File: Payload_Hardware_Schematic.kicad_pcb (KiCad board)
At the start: 2 copper layers, 109 x 54.5 mm, 10 parts, among them J1 Micro_SD_Card, J2 Conn_01x02_Socket, J3 Conn_01x04_Pin, J4 Conn_01x02, J5 Conn_01x04_Pin, U1 STM32F411 BlackPill, U2 MPM3610, U4 LSM9DS1, U5 MPM3610, U6 BMP388

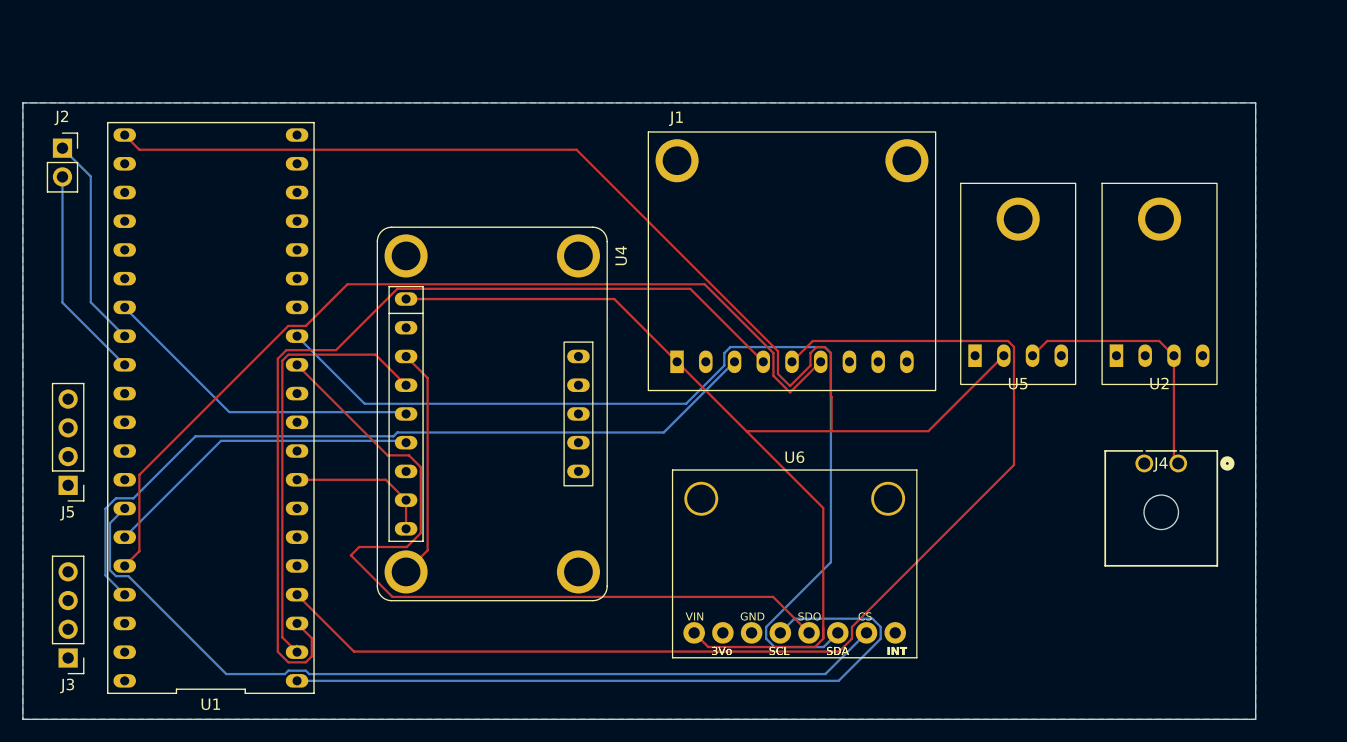
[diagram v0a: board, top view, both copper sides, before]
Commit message: PCB Layout 2
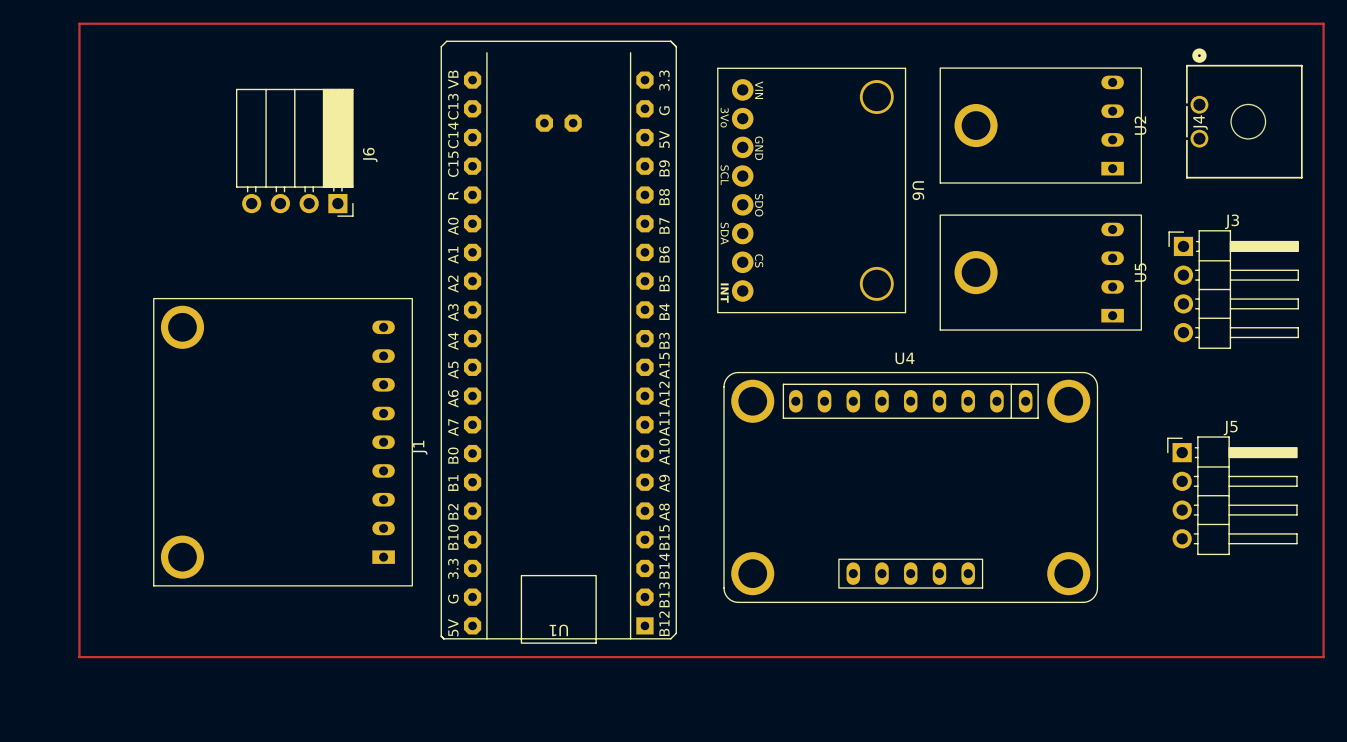
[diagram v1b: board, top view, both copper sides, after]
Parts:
- removed J2: Conn_01x02_Socket, Connector_PinSocket_2.54mm:PinSocket_1x02_P2.54mm_Vertical
- added J6: Conn_01x04_Socket, Connector_PinSocket_2.54mm:PinSocket_1x04_P2.54mm_Horizontal, F.Cu at (92.8, 56.4)
- J3, J5: footprint Connector_PinHeader_2.54mm:PinHeader_1x04_P2.54mm_Vertical -> Connector_PinHeader_2.54mm:PinHeader_1x04_P2.54mm_Horizontal
- U1: footprint Avionics_Symbols:STM32F411 -> Payload-STM32:STM32F411_Black_Pill
- moved J3 105.1 mm to (167.6, 60.2), turned to 0 degrees
- moved J5 98.5 mm to (167.5, 78.4), turned to 0 degrees
- moved U4 44.6 mm to (143.5, 73.9), turned to 180 degrees
- moved J1 36.8 mm to (96.9, 77.5), turned to 90 degrees
- moved U6 33.1 mm to (134.7, 55.2), turned to -90 degrees
- moved J4 31.8 mm to (169.0, 47.7), turned to 90 degrees
- moved U1 31.1 mm to (112.4, 69.6), turned to 180 degrees
- moved U2 20.8 mm to (161.3, 49.5), turned to 90 degrees
- moved U5 11.1 mm to (161.3, 62.5), turned to 90 degrees
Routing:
- net /<NO NET>: track 176.9 -> 0.00 mm
- net /MOSI2: track 104.0 -> 0.00 mm
- net /MOSI3: track 87.4 -> 0.00 mm
- net /NSS2: track 82.1 -> 0.00 mm
- net /MISO2: track 81.1 -> 0.00 mm
- net /NSS3: track 78.4 -> 0.00 mm
- net /MISO3: track 71.1 -> 0.00 mm
- net /SCK2: track 69.3 -> 0.00 mm
- net /SCK3: track 63.9 -> 0.00 mm
- net /SCK4: track 39.2 -> 0.00 mm
- net /MOSI4: track 28.8 -> 0.00 mm
- net /CSIMU: track 28.5 -> 0.00 mm
- net /7.2V: track 23.3 -> 0.00 mm
- net /GND: track 20.9 -> 0.00 mm
- net /UART_TX: track 18.9 -> 0.00 mm
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- removed copper zone on B.Cu, net (none)
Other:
- board outline removed
- board text removed: "3Vo"
- board text removed: "INT"
- board text removed: "SCL"
- board text removed: "SDA"
